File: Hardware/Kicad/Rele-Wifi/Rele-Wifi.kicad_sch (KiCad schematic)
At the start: 52 parts, among them J1 ULTRASONIDO, J13 Screw_Terminal, Q1 MMBT2222A, Q2 MMBT2222A, Q3 MMBT2222A, Q4 MMBT2222A, SW1 SW_DPST_x2, U1 817C, U2 817C, U3 817C, U4 817C, U5 L7805, U7 ESP32_DevKit_V1_CH9102X

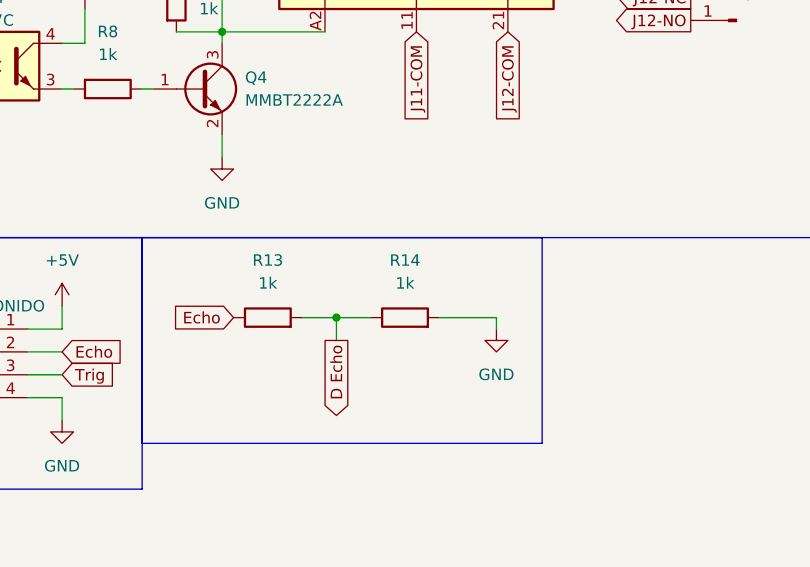
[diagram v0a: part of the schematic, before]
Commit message: A imprimir
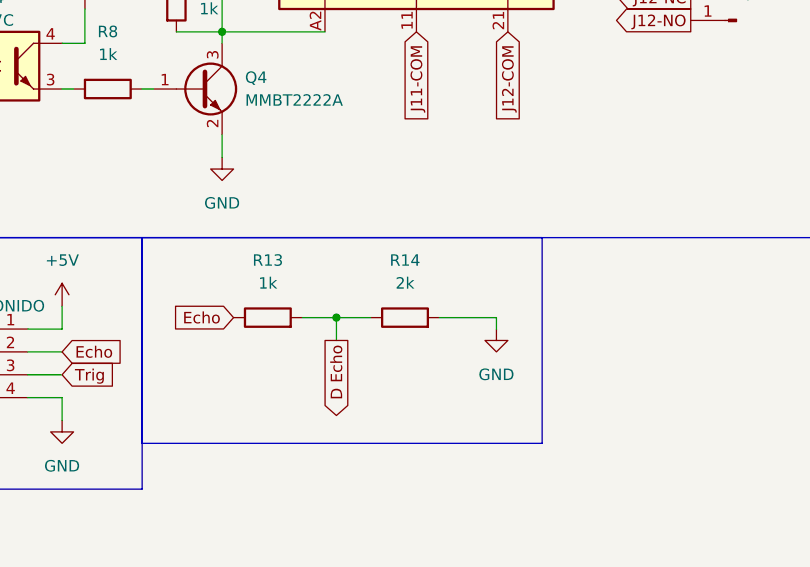
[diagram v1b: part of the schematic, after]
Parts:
- R13: footprint Resistor_THT:R_Axial_DIN0204_L3.6mm_D1.6mm_P7.62mm_Horizontal -> Resistor_SMD:R_0805_2012Metric_Pad1.20x1.40mm_HandSolder
- R14: value 1k -> 2k; footprint Resistor_THT:R_Axial_DIN0204_L3.6mm_D1.6mm_P7.62mm_Horizontal -> Resistor_SMD:R_0805_2012Metric_Pad1.20x1.40mm_HandSolder
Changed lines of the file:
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@@
 			)
 		)
-		(property "Value" "1k"
+		(property "Value" "2k"
 			(at 229.87 119.38 90)
 			(effects
@@
 			)
 		)
-		(property "Footprint" "Resistor_THT:R_Axial_DIN0204_L3.6mm_D1.6mm_P7.62mm_Horizontal"
+		(property "Footprint" "Resistor_SMD:R_0805_2012Metric_Pad1.20x1.40mm_HandSolder"
 			(at 229.87 124.968 90)
 			(effects
@@
 			)
 		)
-		(property "Footprint" "Resistor_THT:R_Axial_DIN0204_L3.6mm_D1.6mm_P7.62mm_Horizontal"
+		(property "Footprint" "Resistor_SMD:R_0805_2012Metric_Pad1.20x1.40mm_HandSolder"
 			(at 214.63 124.968 90)
 			(effects
